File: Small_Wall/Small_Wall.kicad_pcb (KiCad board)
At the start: 2 copper layers, 110 x 14.6 mm, 41 parts, among them J1 Conn_01x03, J2 Conn_01x03, J4 Conn_01x03, J5 Conn_01x03, U1 IN-PI55TATPRPGPB, U2 IN-PI55TATPRPGPB, U3 IN-PI55TATPRPGPB, U4 IN-PI55TATPRPGPB, U5 IN-PI55TATPRPGPB, U6 IN-PI55TATPRPGPB, U7 IN-PI55TATPRPGPB

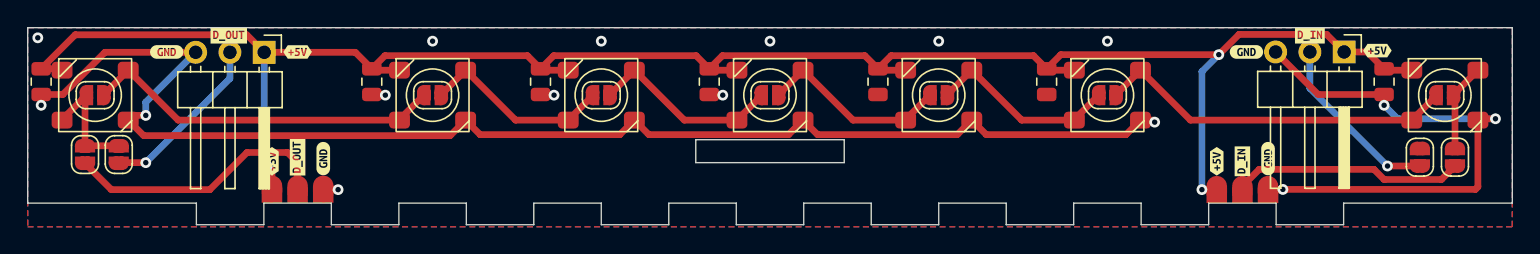
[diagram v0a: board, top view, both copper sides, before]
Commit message: [SMA][WALL] Update wall
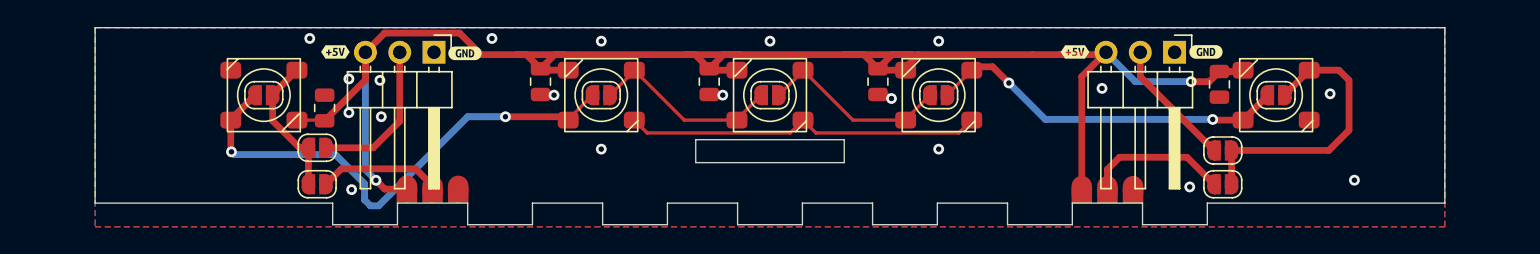
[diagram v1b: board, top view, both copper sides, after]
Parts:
- removed the C1 at (120.5, 101.0)
- removed C7: 100nF, Capacitor_SMD:C_0805_2012Metric
- removed JP10: SolderJumper_2_Open, Jumper:SolderJumper-2_P1.3mm_Open_RoundedPad1.0x1.5mm
- removed the JP4 at (125.0, 102.0)
- removed the U1 at (125.0, 102.0)
- removed U7: IN-PI55TATPRPGPB, LED_SMD:IN-PI55TATPRPGPB
- removed the kibuzzard-64B1960B at (41.9, 106.7)
- removed the kibuzzard-64B1960B at (111.9, 106.7)
- removed the kibuzzard-64B19658 at (108.1, 106.9)
- removed the kibuzzard-64B19658 at (40.0, 98.8)
- removed kibuzzard-64B196A7 (x2): G***, kibuzzard-64B196A7
- removed kibuzzard-64B196D3 (x2): G***, kibuzzard-64B196D3
- moved kibuzzard-64B19658 22.4 mm to (97.6, 98.8)
- moved kibuzzard-64B1960B 22.1 mm to (52.4, 98.9)
- moved JP9 17.3 mm to (41.5, 108.6), turned to 180 degrees
- moved JP2 17.3 mm to (108.5, 108.6), turned to 0 degrees
- moved JP8 14.7 mm to (41.5, 105.9), turned to 180 degrees
- moved JP1 14.6 mm to (108.5, 106.1), turned to 0 degrees
- moved C1 12.8 mm to (108.3, 101.2)
- moved J3 12.6 mm to (50.1, 98.8)
- moved J1 12.6 mm to (105.0, 98.8)
- moved JP3 12.5 mm to (112.5, 102.0)
- moved JP7 12.5 mm to (37.5, 102.0), turned to 0 degrees
- moved U1 12.5 mm to (112.5, 102.0)
- moved U5 12.5 mm to (37.5, 102.0), turned to 180 degrees
- moved J2 10.0 mm to (100.0, 110.0)
- moved J4 10.0 mm to (50.0, 110.0)
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- renumbered C2 to C1, C3 to C2, C4 to C3, C5 to C4, C6 to C5, J4 to J3, J5 to J4, JP5 to JP3, JP6 to JP4, JP7 to JP5, JP8 to JP6, JP9 to JP7, JP11 to JP8, JP12 to JP9, U2 to U1, U3 to U2, U4 to U3, U5 to U4, U6 to U5
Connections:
- J1 pad 1: VDD -> GND
- J1 pad 3: GND -> VDD
- J3 pad 1: VDD -> GND
- J3 pad 3: GND -> VDD
- JP3 pad 1: Net-(JP4-B) (its old number) -> Net-(JP1-B)
- JP7 pad 2: Net-(JP10-A) -> Net-(JP7-B)
- JP8 pad 2: Net-(JP10-B) -> Net-(JP7-B)
- JP9 pad 2: Net-(JP10-B) -> Net-(JP7-B)
- U1 pad 4: Net-(JP4-B) (its old number) -> Net-(JP1-B)
- U5 pad 2: Net-(JP10-A) -> Net-(JP7-B)
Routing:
- net GND: track 146.7 -> 29.7 mm, vias 16 -> 19
- net Net-(JP10-A): track 26.8 -> 0.00 mm
- net Net-(JP4-B) (its old number): track 26.8 -> 0.00 mm
- net Net-(JP6-B): track 14.3 -> 37.7 mm, vias 0 -> 2
- net VDD: track 143.1 -> 122.5 mm, vias 3 -> 2
- net Net-(JP1-B): track 6.59 -> 21.4 mm
- net Net-(JP3-B): track 14.3 -> 27.0 mm, vias 0 -> 2
- net Net-(J4-Pin_2): track 20.0 -> 9.13 mm
- net Net-(JP7-B): track 0.00 -> 10.7 mm
- net Net-(JP10-B): track 8.89 -> 0.00 mm
- net Net-(J2-Pin_2): track 17.2 -> 10.6 mm
- net Net-(J1-Pin_2): track 13.2 -> 9.54 mm, vias 1 -> 0
- net Net-(J3-Pin_2): track 12.8 -> 11.4 mm, vias 1 -> 0
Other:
- board size 110 x 14.6 mm -> 100 x 14.6 mm
